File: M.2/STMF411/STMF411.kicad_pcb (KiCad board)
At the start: 2 copper layers, 22 x 26 mm, 26 parts, among them M1 M.2_Key_E, Q1 2N7002, SW1 RESET, U1 XC6206P332MR, U2 STM32F411CCUx, Y1 16 MHz

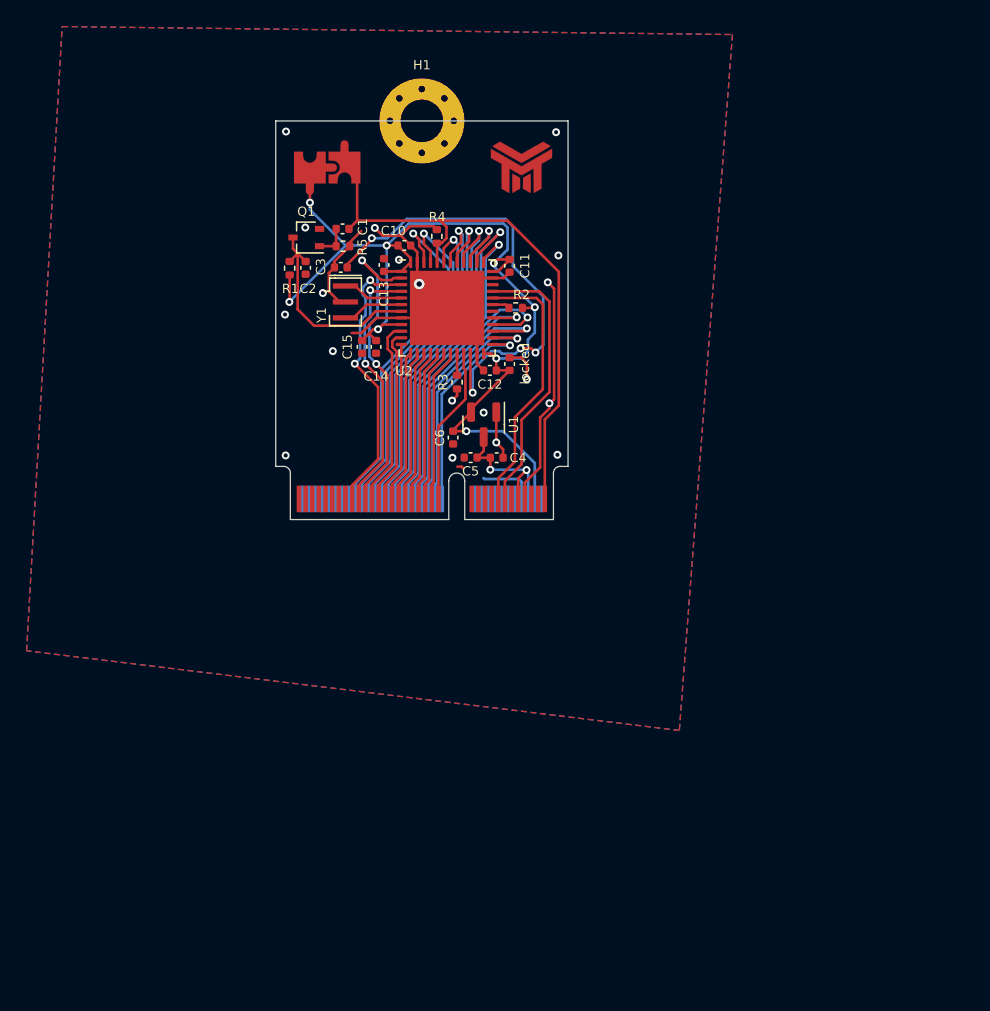
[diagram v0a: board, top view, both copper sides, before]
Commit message: prettify files a lil bit
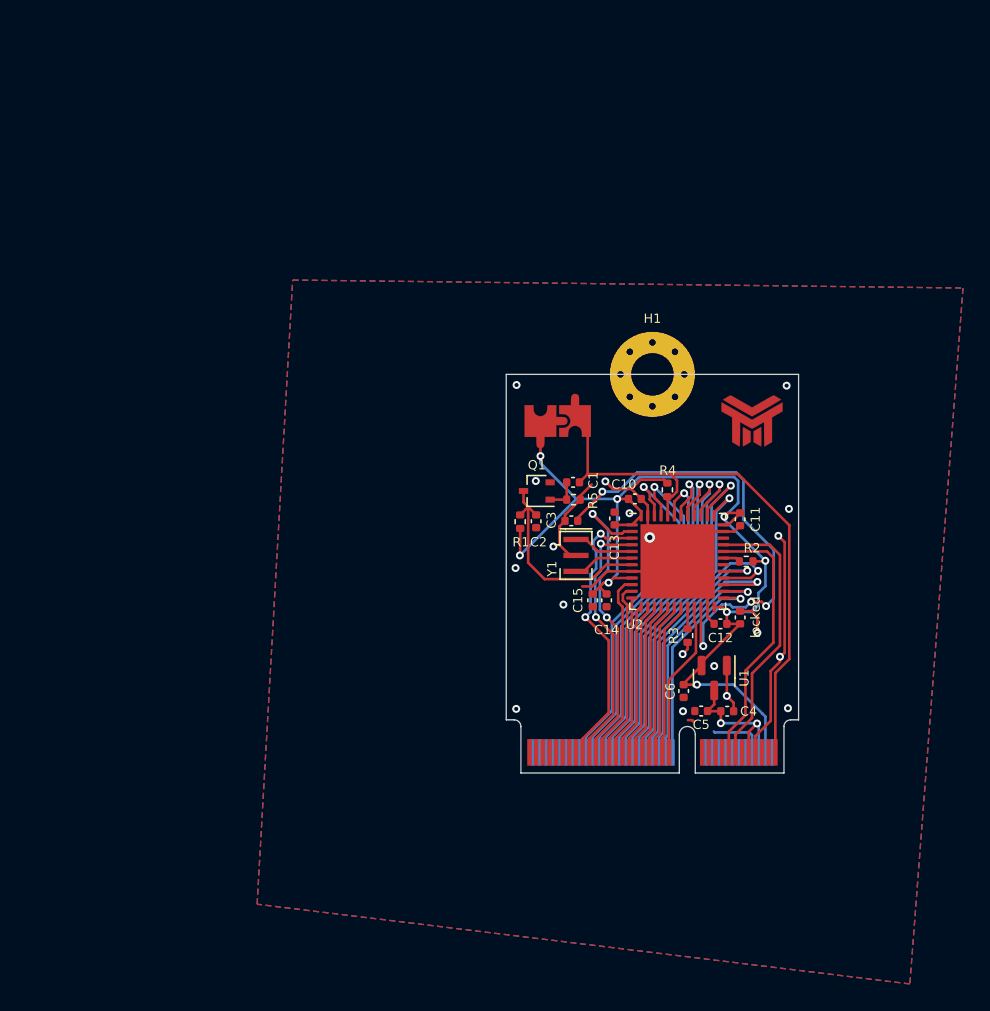
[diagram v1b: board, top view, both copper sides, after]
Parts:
- moved C10 25.8 mm to (27.0, 28.4)
- moved C11 25.8 mm to (34.9, 30.0)
- moved C12 25.8 mm to (33.5, 37.9)
- moved C13 25.8 mm to (25.5, 29.9)
- moved C15 25.8 mm to (23.9, 36.1)
- moved C2 25.8 mm to (19.6, 30.1)
- moved C3 25.8 mm to (22.2, 30.1)
- moved C5 25.8 mm to (32.0, 44.4)
- moved C6 25.8 mm to (30.7, 42.9)
- moved H1 25.8 mm to (28.4, 19.1)
- moved L1 25.8 mm to (35.9, 22.6)
- moved M1 25.8 mm to (28.4, 49.1)
- moved Q1 25.8 mm to (19.6, 27.9)
- moved R1 25.8 mm to (18.4, 30.2)
- moved R3 25.8 mm to (31.0, 38.7)
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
